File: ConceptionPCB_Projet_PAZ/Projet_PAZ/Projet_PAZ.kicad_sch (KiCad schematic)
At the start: 52 parts, among them IC2 STM32L412KBT6, J1 Conn_01x02, J13 Conn_01x02, J9 Conn_02x07_Odd_Even, Q3 2N2219, Q5 Q_Photo_NPN, U4 BU33SD5WG-TR

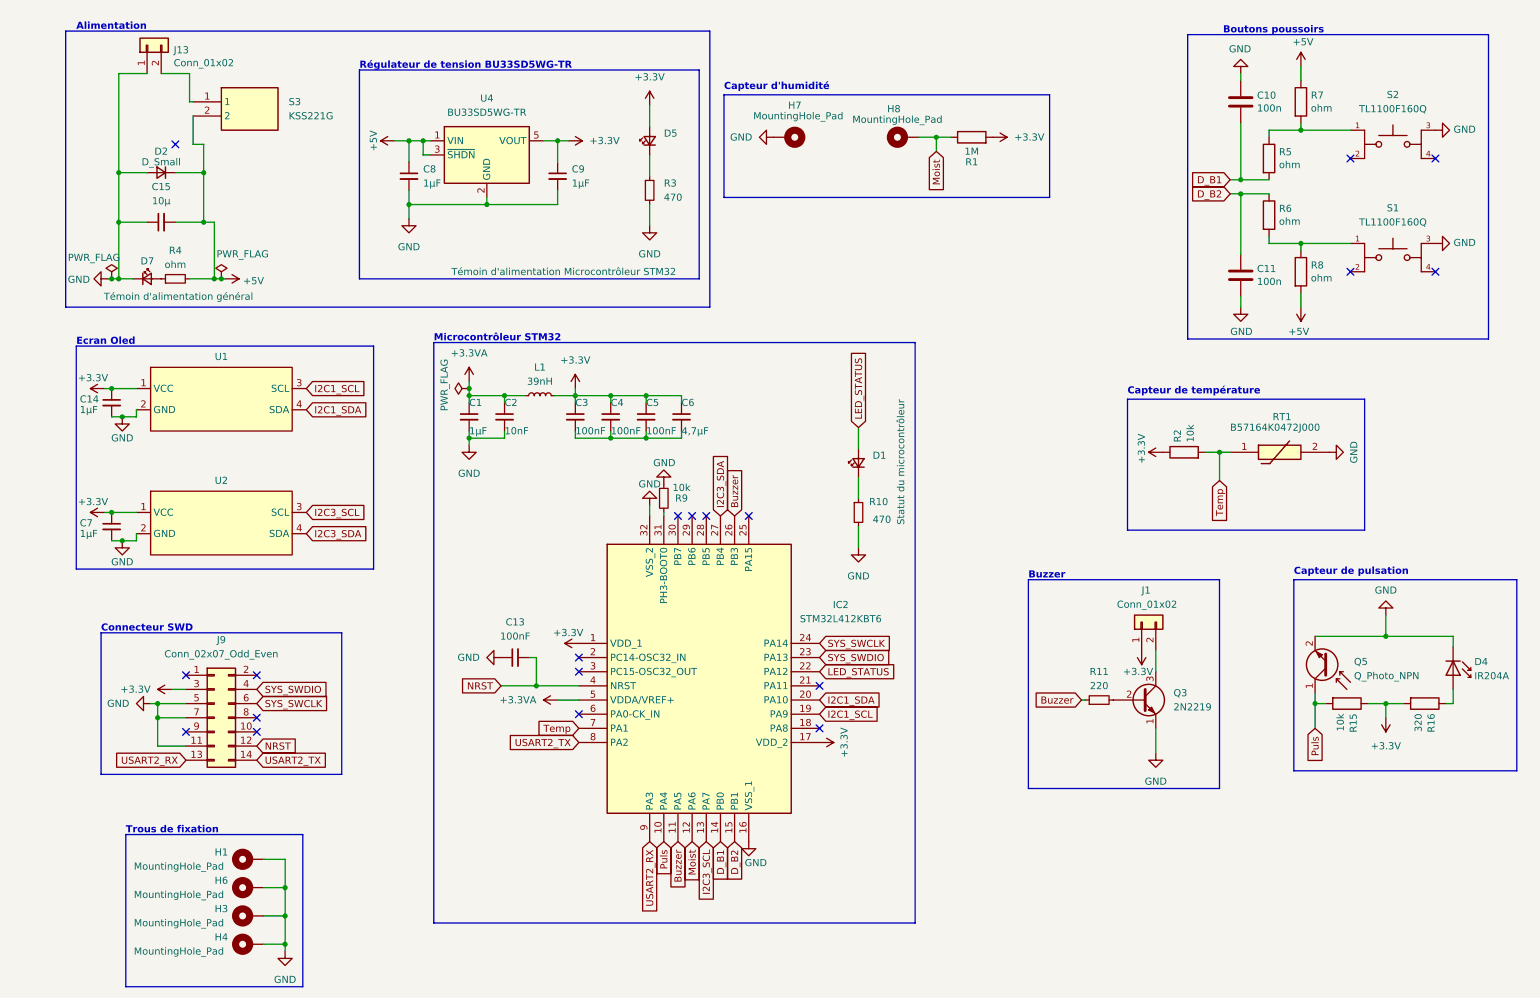
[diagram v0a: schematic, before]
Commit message: Add files via upload
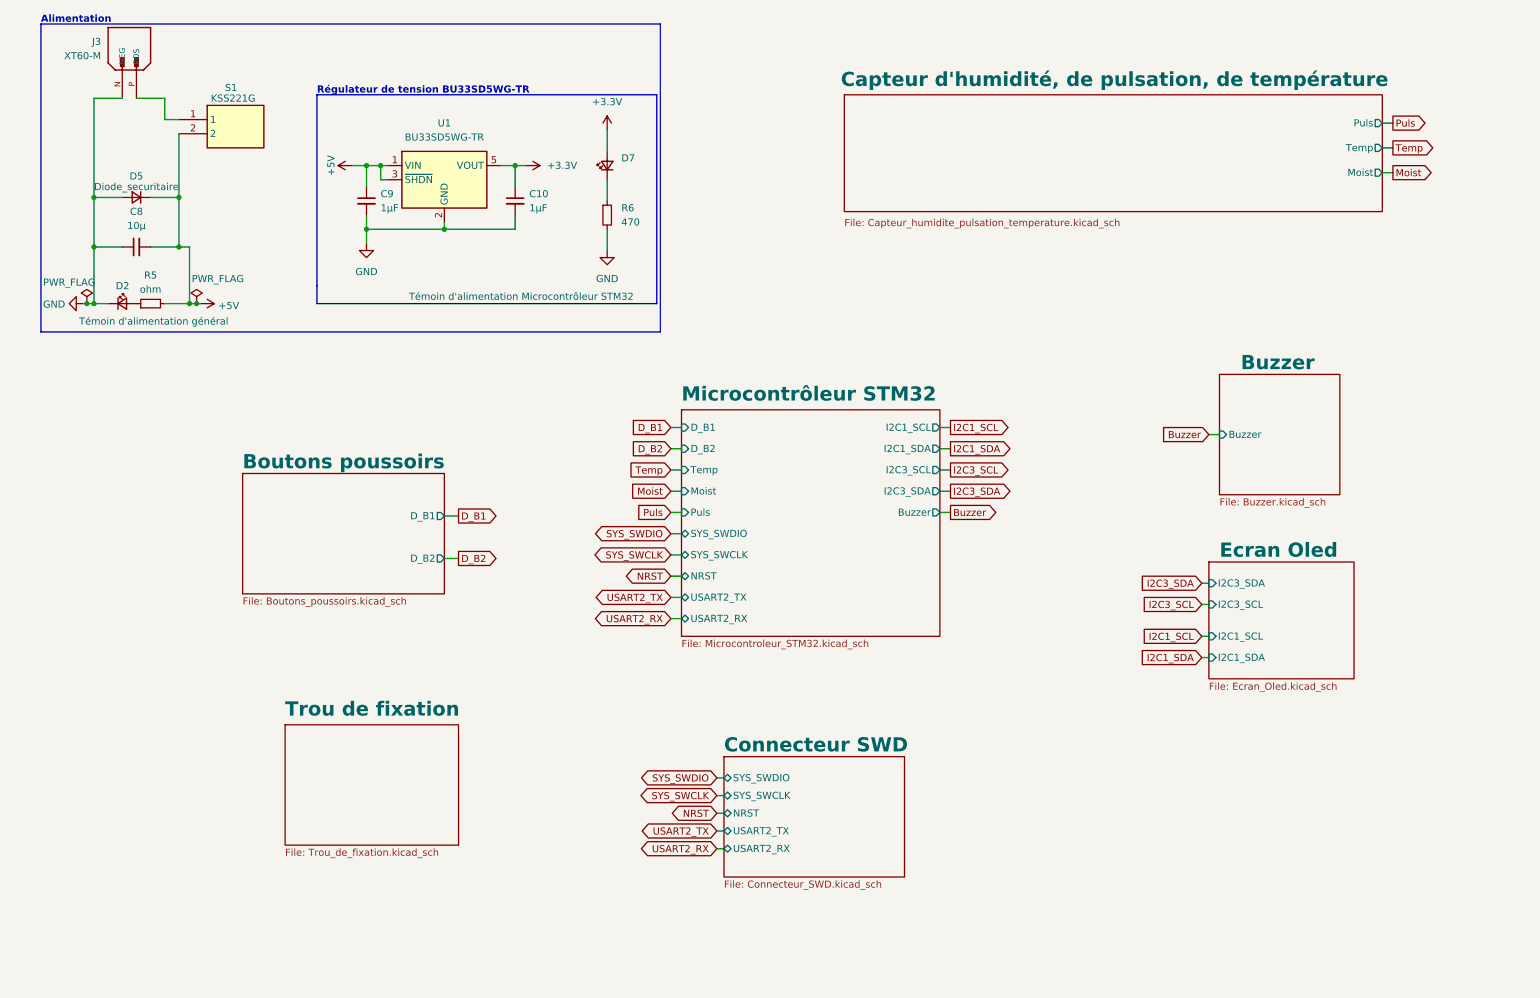
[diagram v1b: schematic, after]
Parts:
- removed C1, C14, C7: 1µF, Capacitor_SMD:C_0603_1608Metric_Pad1.08x0.95mm_HandSolder, symbol Device:C_Small
- removed C10, C11: 100n, Capacitor_SMD:C_0603_1608Metric_Pad1.08x0.95mm_HandSolder, symbol Device:C
- removed C13, C3, C4, C5: 100nF, Capacitor_SMD:C_0603_1608Metric_Pad1.08x0.95mm_HandSolder, symbol Device:C_Small
- removed C15: 10µ, Capacitor_SMD:C_0603_1608Metric_Pad1.08x0.95mm_HandSolder, symbol Device:C_Small
- removed C2: 10nF, Capacitor_SMD:C_0603_1608Metric_Pad1.08x0.95mm_HandSolder, symbol Device:C_Small
- removed C6: 4,7µF, Capacitor_SMD:C_0603_1608Metric_Pad1.08x0.95mm_HandSolder, symbol Device:C_Small
- removed D1: Statut du microcontrôleur, LED_SMD:LED_0603_1608Metric_Pad1.05x0.95mm_HandSolder, symbol Device:LED_Small
- removed D2: D_Small, LED_SMD:LED_0603_1608Metric_Pad1.05x0.95mm_HandSolder, symbol Device:D_Small
- removed D4: IR204A, LED_THT:LED_D3.0mm_IRBlack, symbol LED:IR204A
- removed D5: Témoin d'alimentation Microcontrôleur STM32, LED_SMD:LED_0603_1608Metric_Pad1.05x0.95mm_HandSolder, symbol Device:LED_Small
- removed H1, H3, H4, H6, H7, H8: MountingHole_Pad, MountingHole:MountingHole_3.2mm_M3_DIN965_Pad, symbol Mechanical:MountingHole_Pad
- removed IC2: STM32L412KBT6, MesEmpreintes:QFP80P900X900X160-32N, symbol STM32L412KBT6:STM32L412KBT6
- removed J1: Conn_01x02, symbol Connector_Generic:Conn_01x02
- removed J13: Conn_01x02, Connecteur_alimentation:connecteur, symbol Connector_Generic:Conn_01x02
- removed J9: Conn_02x07_Odd_Even, Connector_PinHeader_1.27mm:PinHeader_2x07_P1.27mm_Vertical_SMD, symbol Connector_Generic:Conn_02x07_Odd_Even
- removed L1: 39nH, Inductor_SMD:L_0603_1608Metric_Pad1.05x0.95mm_HandSolder, symbol Device:L_Small
- removed Q3: 2N2219, Package_TO_SOT_THT:TO-39-3, symbol Transistor_BJT:2N2219
- removed Q5: Q_Photo_NPN, symbol Device:Q_Photo_NPN
- removed R1: 1M, Resistor_SMD:R_0603_1608Metric_Pad0.98x0.95mm_HandSolder, symbol Device:R
- removed R10, R3: 470, Resistor_SMD:R_0603_1608Metric_Pad0.98x0.95mm_HandSolder, symbol Device:R_Small
- removed R11: 220, Resistor_SMD:R_0603_1608Metric_Pad0.98x0.95mm_HandSolder, symbol Device:R_Small
- removed R15, R2: 10k, Resistor_SMD:R_0603_1608Metric_Pad0.98x0.95mm_HandSolder, symbol Device:R
- removed R16: 320, Resistor_SMD:R_0603_1608Metric_Pad0.98x0.95mm_HandSolder, symbol Device:R
- removed R4: ohm, Resistor_SMD:R_0603_1608Metric_Pad0.98x0.95mm_HandSolder, symbol Device:R_Small
- removed R5, R6, R7, R8: ohm, Resistor_SMD:R_0603_1608Metric_Pad0.98x0.95mm_HandSolder, symbol Device:R
- removed R9: 10k, Resistor_SMD:R_0603_1608Metric_Pad0.98x0.95mm_HandSolder, symbol Device:R_Small
- removed RT1: B57164K0472J000, MesEmpreintes:B57164K_K164, symbol B57164K0472J000:B57164K0472J000
- removed S1, S2: TL1100F160Q, MesEmpreintes:SW_TL1100F160Q, symbol TL1100F160Q:TL1100F160Q
- removed S3: KSS221G, MesEmpreintes:KSS221G, symbol KSS221G:KSS221G
- removed U1, U2: ~, symbol MesSymboles:MDOB128064WV-YBI
- removed U4: BU33SD5WG-TR, Package_TO_SOT_SMD:SOT-23-5, symbol Regulator_Linear:MCP1802x-xx02xOT
- added C10: 1µF, Capacitor_SMD:C_0603_1608Metric_Pad1.08x0.95mm_HandSolder, symbol Device:C_Small
- added D2: Témoin d'alimentation général, LED_SMD:LED_0603_1608Metric_Pad1.05x0.95mm_HandSolder, symbol Device:LED_Small
- added D5: Diode_securitaire, Diode_SMD:D_0603_1608Metric_Pad1.05x0.95mm_HandSolder, symbol Device:D_Small
- added J3: XT60-M, MesEmpreintes:AMASS_XT60-M, symbol XT60-M:XT60-M
- added R5: ohm, Resistor_SMD:R_0603_1608Metric_Pad0.98x0.95mm_HandSolder, symbol Device:R_Small
- added R6: 470, Resistor_SMD:R_0603_1608Metric_Pad0.98x0.95mm_HandSolder, symbol Device:R_Small
- added S1: KSS221G, MesEmpreintes:KSS221G, symbol KSS221G:KSS221G
- added U1: BU33SD5WG-TR, Package_TO_SOT_SMD:SOT-23-5, symbol Regulator_Linear:MCP1802x-xx02xOT
- C8: value 1µF -> 10µ
- D7: value Témoin d'alimentation général -> Témoin d'alimentation Microcontrôleur STM32
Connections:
- net +3.3V: now also D7.2 (A), C10.1, U1.5 (VOUT); no longer C9.1
- net +5V: now also C8.2, C9.1, D5.1 (K), R5.2, S1.2, U1.1 (VIN), U1.3 (~{SHDN}); no longer C8.1
- net GND: now also C8.1, C10.2, D2.1 (K), D5.2 (A), J3.N (NEG), R6.2, U1.2 (GND); no longer C8.2, D7.1 (K)
- new net: D2.2 (A), R5.1
- new net: J3.P (POS), S1.1
- new net: D7.1 (K), R6.1
- no-connect marks 19 -> 0
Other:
- added sheet Boutons poussoirs (Boutons_poussoirs.kicad_sch)
- added sheet Buzzer (Buzzer.kicad_sch)
- added sheet Capteur d'humidité, de pulsation, de température (Capteur_humidite_pulsation_temperature.kicad_sch)
- added sheet Connecteur SWD (Connecteur_SWD.kicad_sch)
- added sheet Ecran Oled (Ecran_Oled.kicad_sch)
- added sheet Microcontrôleur STM32 (Microcontroleur_STM32.kicad_sch)
- added sheet Trou de fixation (Trou_de_fixation.kicad_sch)
- note removed: "Boutons poussoirs"
- note removed: "Buzzer"
- note removed: "Capteur d'humidité"
- note removed: "Capteur de pulsation"
- note removed: "Capteur de température"
- note removed: "Connecteur SWD"
- note removed: "Ecran Oled"
- note removed: "Microcontrôleur STM32"
- note removed: "Trous de fixation"
